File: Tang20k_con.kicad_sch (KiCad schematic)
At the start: 1 part

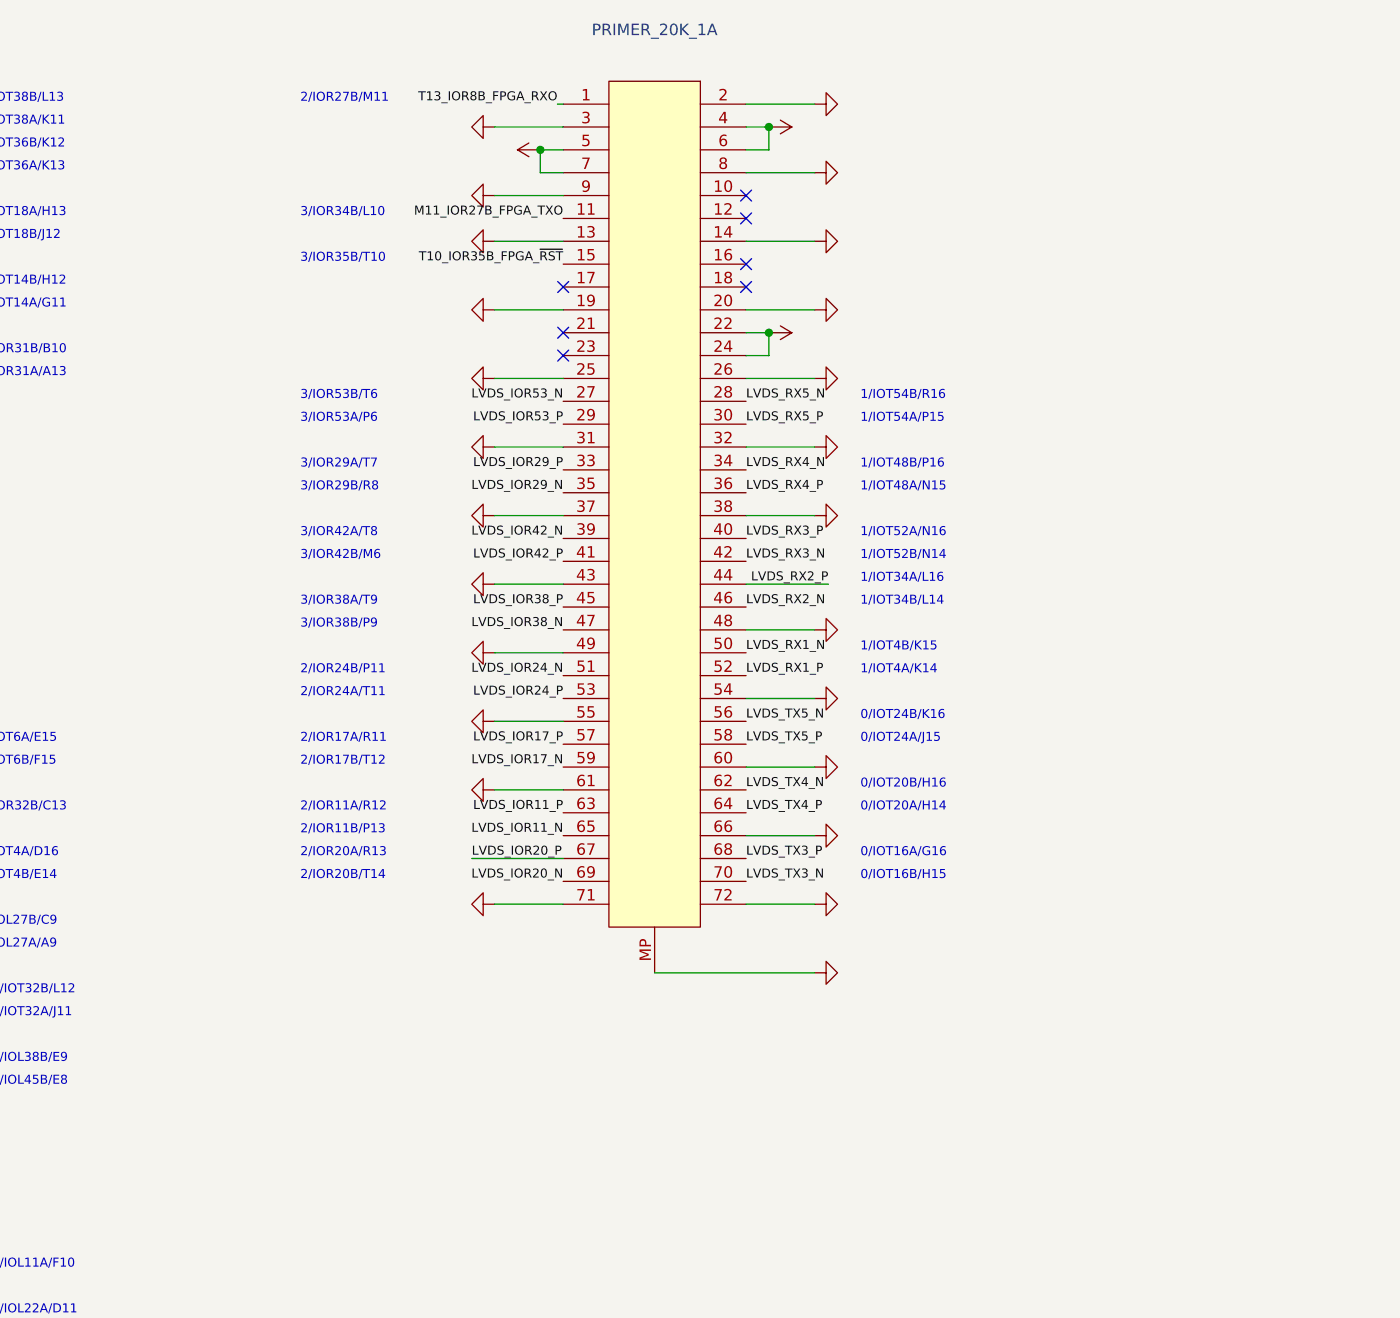
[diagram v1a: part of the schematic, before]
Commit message: WIP
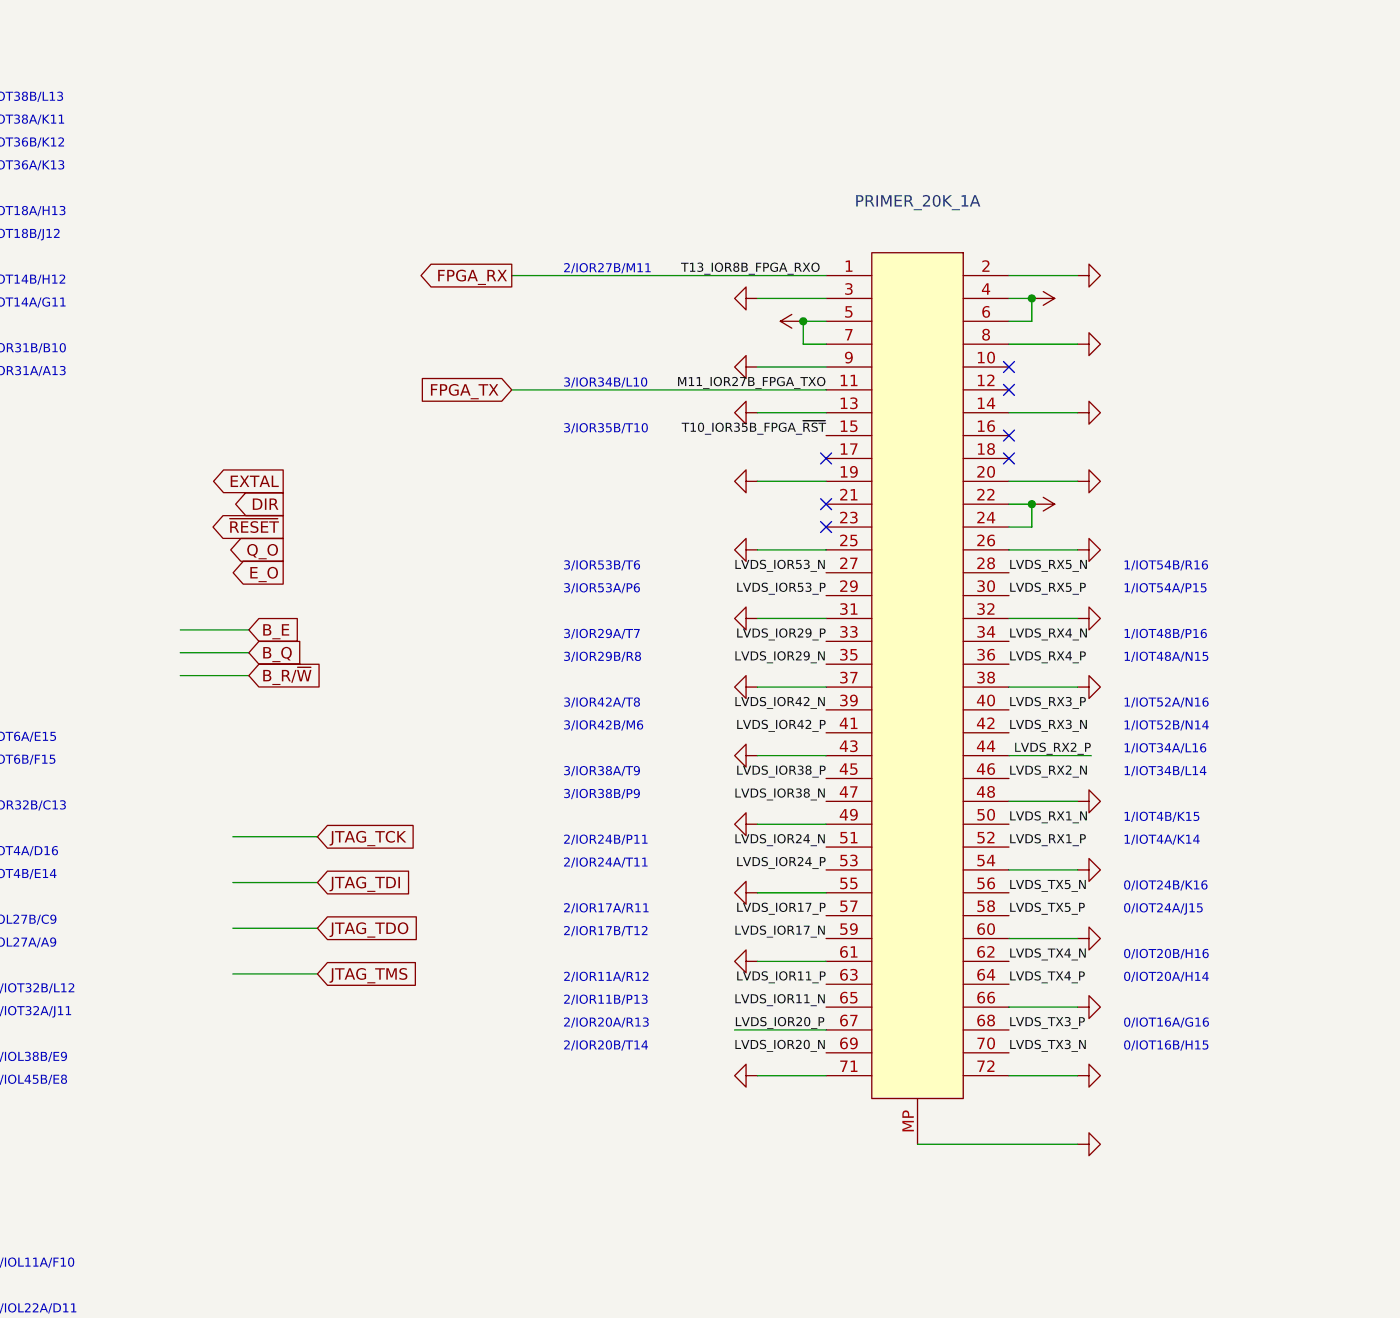
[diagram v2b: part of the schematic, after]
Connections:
- net M11_IOR27B_FPGA_TXO renamed FPGA_TX
- net T13_IOR8B_FPGA_RXO renamed FPGA_RX
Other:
- moved on the sheet: PRIMER_20K_1A

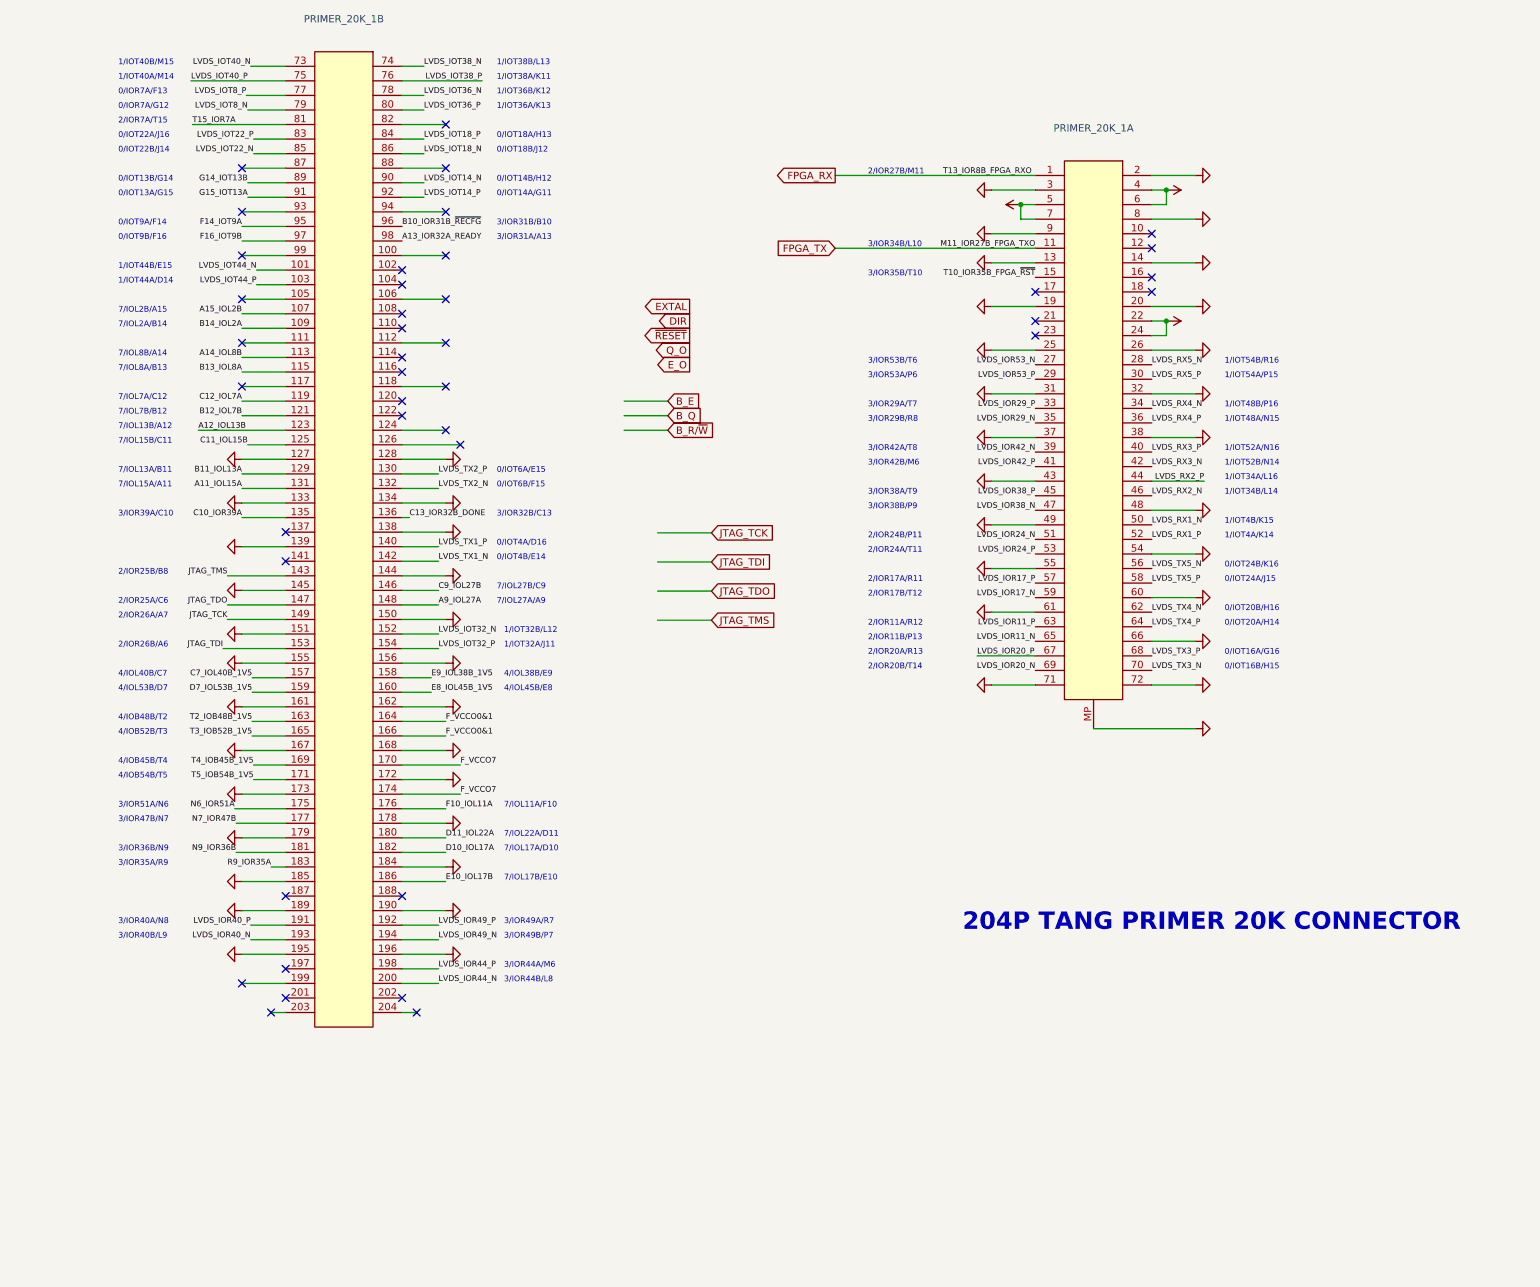
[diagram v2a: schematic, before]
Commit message: wip
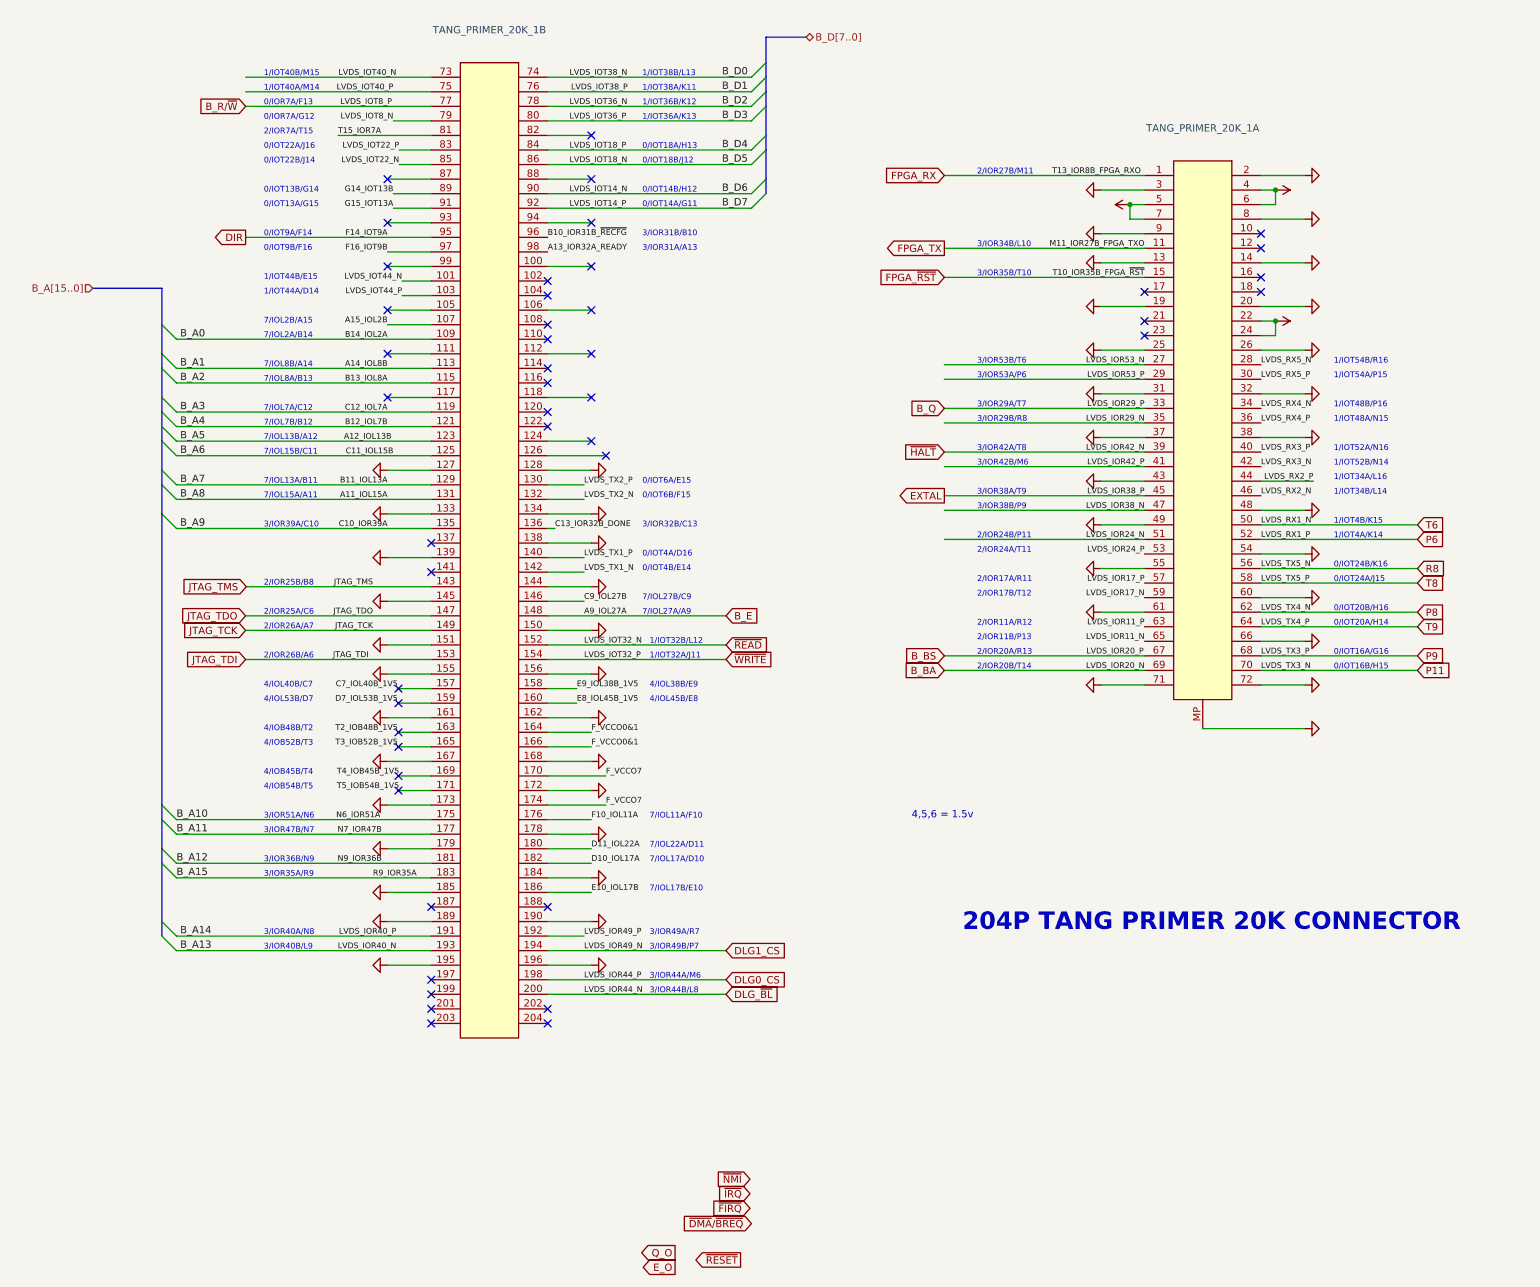
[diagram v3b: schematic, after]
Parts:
- renumbered PRIMER_20K_1 to TANG_PRIMER_20K_1
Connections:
- net A9_IOL27A is gone; now on net B_E: TANG_PRIMER_20K_1.148
- net F14_IOT9A is gone; now on net DIR: TANG_PRIMER_20K_1.95
- net LVDS_IOR29_P is gone; now on net B_Q: TANG_PRIMER_20K_1.33
- net LVDS_IOR38_P is gone; now on net EXTAL: TANG_PRIMER_20K_1.45
- net LVDS_IOT8_P is gone; now on net B_R/~{W}: TANG_PRIMER_20K_1.77
- net C10_IOR39A renamed B_A9
- net C11_IOL15B renamed B_A6
- net C12_IOL7A renamed B_A3
- net LVDS_IOR20_N renamed B_BA
- net LVDS_IOR20_P renamed B_BS
- net LVDS_IOR40_N renamed B_A13
- net LVDS_IOR40_P renamed B_A14
- net LVDS_IOR42_N renamed ~{HALT}
- net LVDS_IOR44_N renamed DLG_~{BL}
- net LVDS_IOR44_P renamed DLG0_CS
- net LVDS_IOR49_N renamed DLG1_CS
- net LVDS_IOT14_N renamed B_D6
- net LVDS_IOT14_P renamed B_D7
- net LVDS_IOT18_N renamed B_D5
- net LVDS_IOT18_P renamed B_D4
- net LVDS_IOT32_N renamed ~{READ}
- net LVDS_IOT32_P renamed ~{WRITE}
- net LVDS_IOT36_N renamed B_D2
- net LVDS_IOT36_P renamed B_D3
- net LVDS_IOT38_N renamed B_D0
- net LVDS_IOT38_P renamed B_D1
- net LVDS_RX1_N renamed T6
- net LVDS_RX1_P renamed P6
- net LVDS_TX3_N renamed P11
- net LVDS_TX3_P renamed P9
- net LVDS_TX4_N renamed P8
- net LVDS_TX4_P renamed T9
- net LVDS_TX5_N renamed R8
- net LVDS_TX5_P renamed T8
- net N6_IOR51A renamed B_A10
- net N7_IOR47B renamed B_A11
- net N9_IOR36B renamed B_A12
- net R9_IOR35A renamed B_A15
- net T10_IOR35B_FPGA_~{RST} renamed FPGA_~{RST}
- no-connect marks 40 -> 46
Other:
- note added: "4,5,6 = 1.5v"
- moved on the sheet: TANG_PRIMER_20K_1A, TANG_PRIMER_20K_1B
